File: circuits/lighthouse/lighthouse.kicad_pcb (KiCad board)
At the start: 2 copper layers, 84 x 112 mm, 83 parts, among them IC1 SX1308, J1 USB_C_Receptacle_PowerOnly_6P, J2 USB_B_Micro, Q1 S9013, Q2 FS8205A, Q3 2N7002K, Q4 SS8050, Q5 SS8050, U1 R300, U10 CP2102-GMR, U2 AMS1117-3.3, U4 TP4056-42-ESOP8, U5 DW01A, U6 AMS1117-3.3, U7 ESP32-WROOM-32

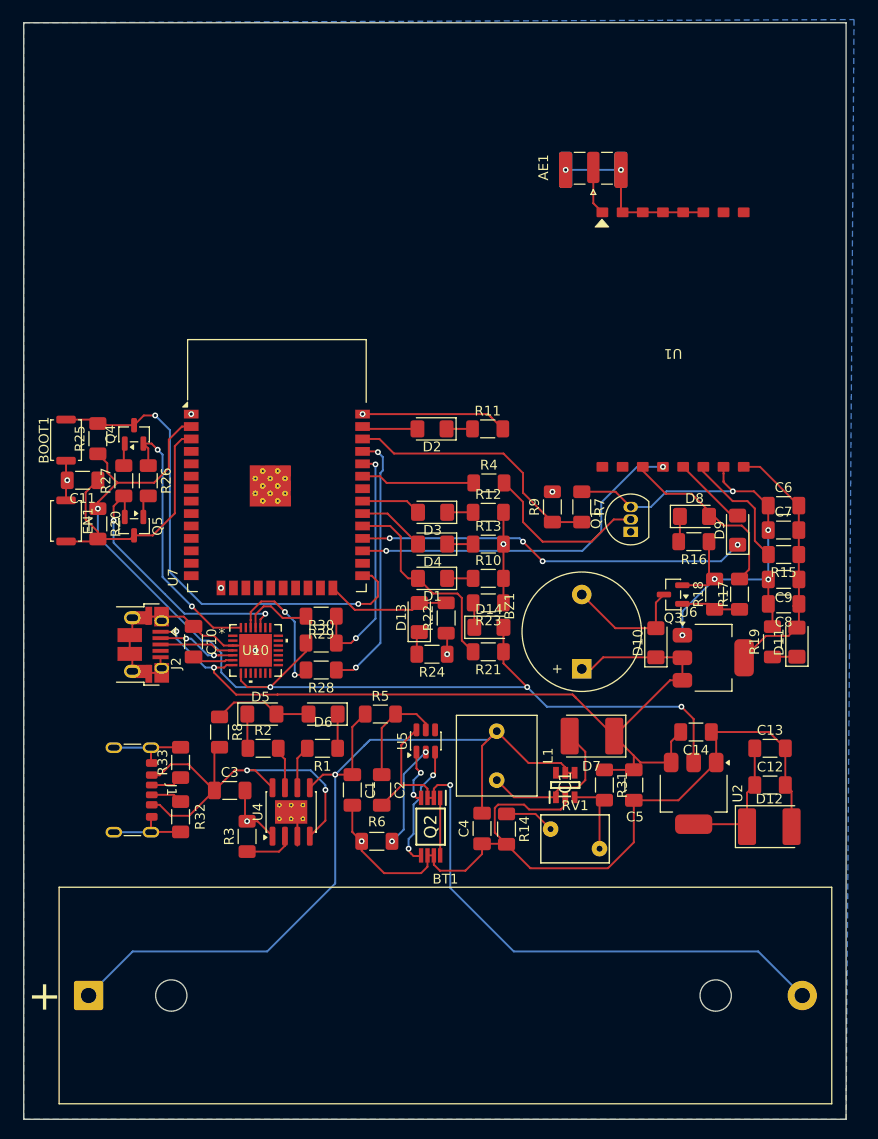
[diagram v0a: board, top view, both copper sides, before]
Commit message: Rewamped the pcb
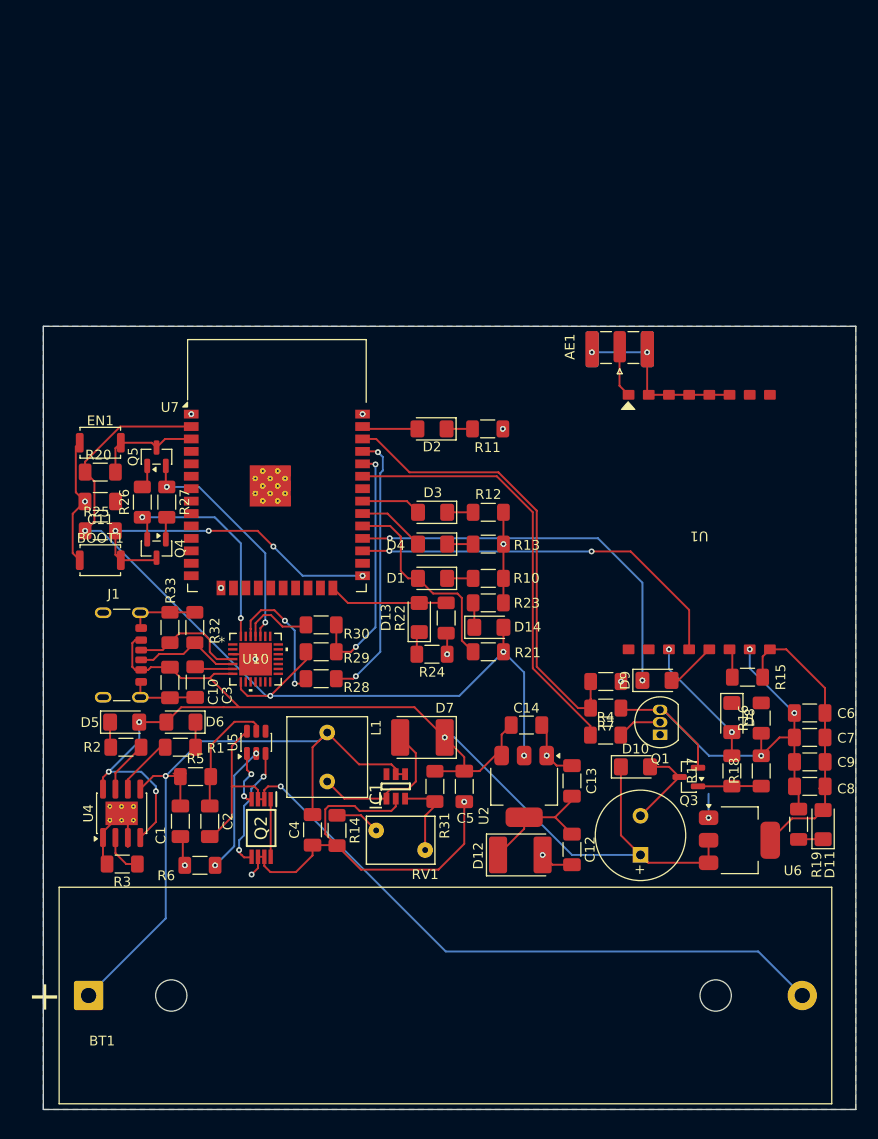
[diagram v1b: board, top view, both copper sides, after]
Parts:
- removed J2: USB_B_Micro, Connector_USB:USB_Micro-B_Amphenol_10103594-0001LF_Horizontal
- removed R8: 2, Resistor_SMD:R_1206_3216Metric_Pad1.30x1.75mm_HandSolder
- BZ1: footprint Buzzer_Beeper:Buzzer_12x9.5RM7.6 -> Buzzer_Beeper:MagneticBuzzer_PUI_AT-0927-TT-6-R
- C4, C5: value C -> 10u
- J1: value USB_C_Receptacle_PowerOnly_6P -> USB_C_Receptacle_6P
- moved R4 28.4 mm to (91.4, 105.8)
- moved D12 25.6 mm to (82.7, 118.0)
- moved C6 21.4 mm to (112.3, 103.5)
- moved C7 21.4 mm to (112.3, 106.0)
- moved C12 21.3 mm to (88.0, 117.4), turned to -90 degrees
- moved Q1 20.9 mm to (97.0, 105.7)
- moved D8 20.9 mm to (104.3, 104.0), turned to -90 degrees
- moved R7 20.7 mm to (91.5, 103.0), turned to 180 degrees
- moved C13 20.5 mm to (88.0, 110.4), turned to 90 degrees
- moved R5 19.9 mm to (49.5, 110.0)
- moved BZ1 19.9 mm to (95.0, 118.0)
- moved R32 19.4 mm to (49.5, 94.8), turned to 90 degrees
- moved R16 19.3 mm to (107.3, 104.0), turned to 90 degrees
- moved D11 18.8 mm to (113.7, 114.9)
- moved R19 18.8 mm to (111.2, 114.9)
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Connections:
- net Net-(U7-IO22) renamed RFID_PW_SENSE
- C3 pad 1: Net-(U4-CE) -> +5V
- D5 pad 2: Net-(D5-A) -> +5V
- D6 pad 2: Net-(D5-A) -> +5V
- J1 pad A5: Net-(J1-CC1) -> /Charger/D+
- J1 pad A9: Net-(U4-CE) -> +5V
- J1 pad B5: Net-(J1-CC2) -> /Charger/D-
- J1 pad B9: Net-(U4-CE) -> +5V
- R32 pad 1: Net-(J1-CC2) -> /Charger/D-
- R33 pad 1: Net-(J1-CC1) -> /Charger/D+
- U10 pad 4: Net-(J2-D+) -> /Charger/D+
- U10 pad 5: Net-(J2-D-) -> /Charger/D-
- U4 pad 4: Net-(U4-CE) -> +5V
- U4 pad 8: Net-(U4-CE) -> +5V
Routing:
- net GND: track 167.3 -> 110.8 mm, vias 10 -> 14
- net Net-(U4-CE): track 42.8 -> 0.00 mm, vias 2 -> 0
- net +5V: track 119.8 -> 162.3 mm, vias 2 -> 4
- net RFID_PW: track 11.7 -> 44.1 mm
- net RFID_PW_SENSE: track 27.1 -> 46.7 mm
- net ESP25: track 53.1 -> 34.6 mm, vias 2 -> 4
- net /Charger/+BAT: track 90.7 -> 72.6 mm
- net +3.3V: track 127.7 -> 109.9 mm
- net EN: track 28.2 -> 11.0 mm
- net /Charger/-BAT: track 67.4 -> 81.5 mm
- net Net-(Q1-B): track 18.1 -> 4.57 mm
- net /Charger/D+: track 0.00 -> 11.9 mm
- net /Charger/D-: track 0.00 -> 11.0 mm
- net Net-(D5-A): track 10.2 -> 0.00 mm
- net Net-(U1-EN): track 13.1 -> 3.43 mm
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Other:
- board size 84 x 112 mm -> 83 x 80 mm
